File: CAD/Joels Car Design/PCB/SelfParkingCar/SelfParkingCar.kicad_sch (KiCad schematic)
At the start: 13 parts, among them U1 ESP32-DevKitC

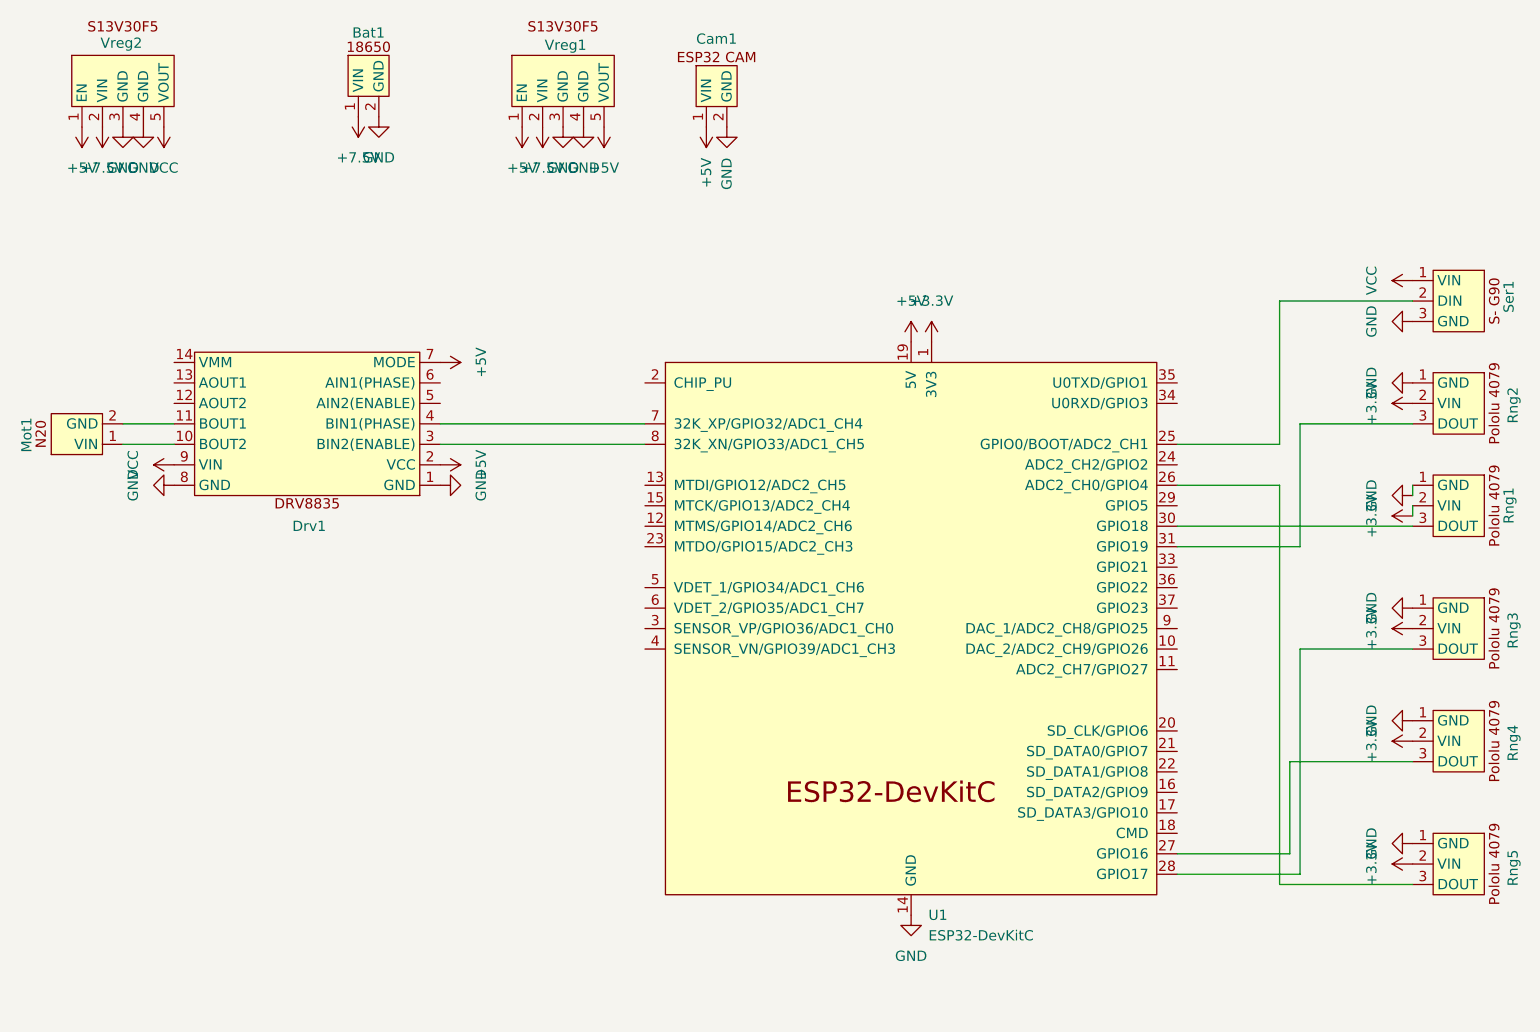
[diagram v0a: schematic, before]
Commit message: PCB Complete
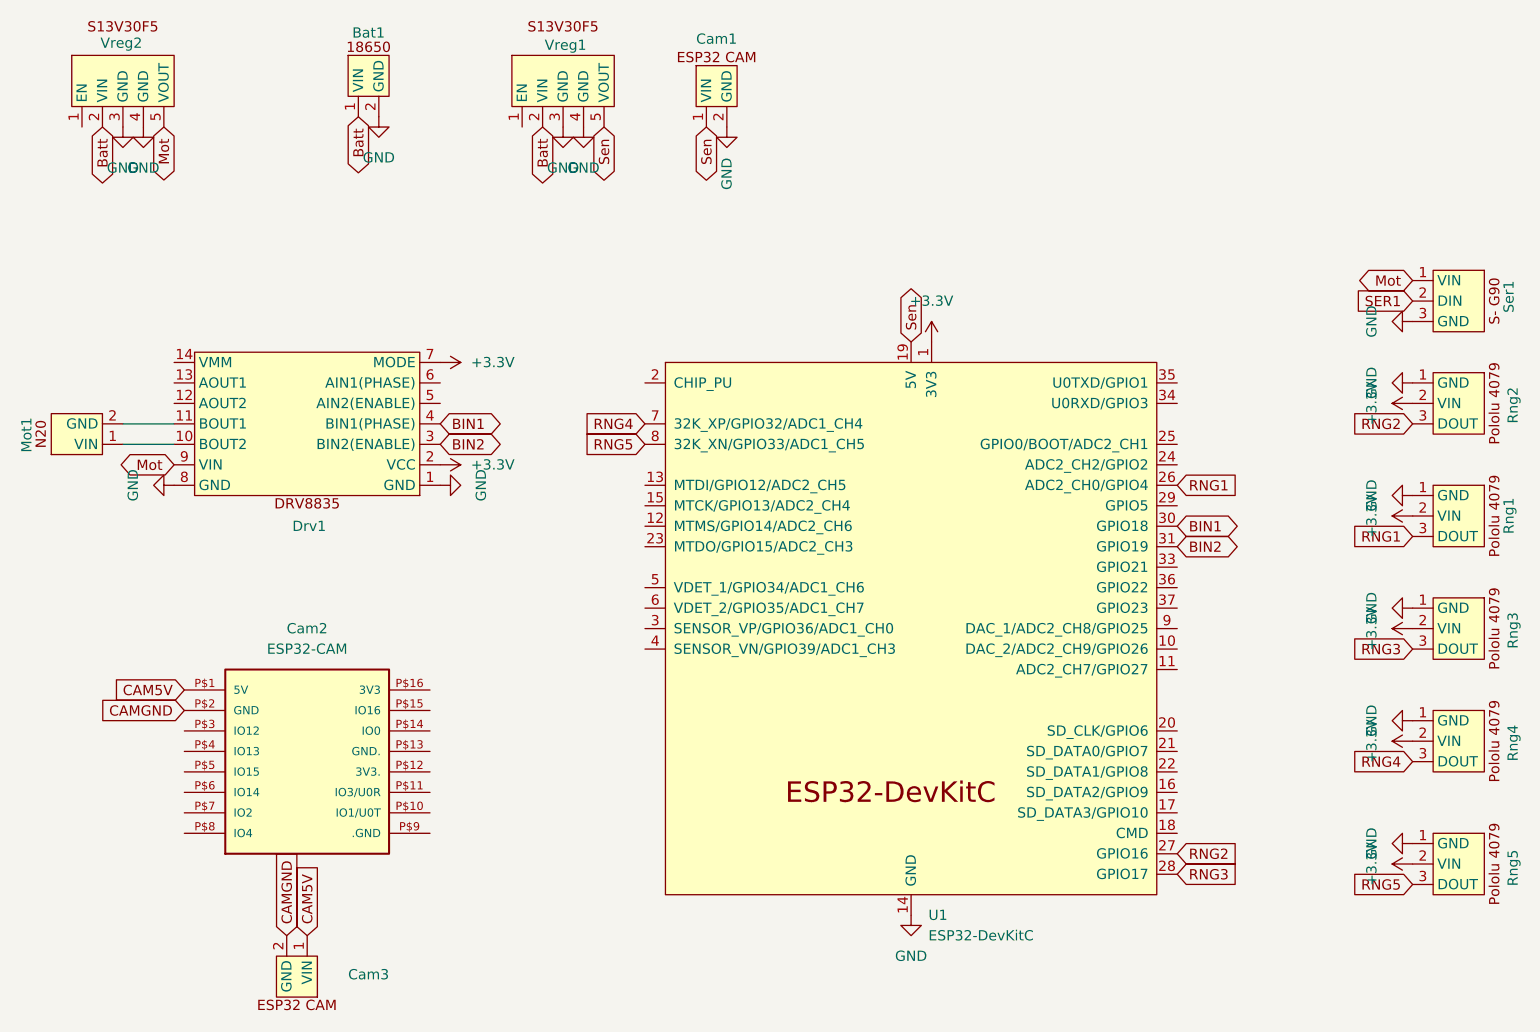
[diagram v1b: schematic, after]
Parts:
- added Cam2: ESP32-CAM, SelfParkingCar:ESP32-CAM, symbol SelfParkingCar:ESP32-CAM
- added Cam3: ~, SelfParkingCar:ESP32 Camera, symbol SelfParkingCar:ESP32 Camera
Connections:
- net +3.3V: now also Drv1.2 (VCC), Drv1.7 (MODE)
- net RNG3: now reaches Rng3.3 (DOUT), U1.28 (GPIO17)
- net at U1.25 (GPIO0/BOOT/ADC2_CH1): no longer Ser1.2 (DIN)
- net RNG1: now reaches U1.26 (ADC2_CH0/GPIO4)
- net RNG1: now also Rng1.3 (DOUT); no longer Rng5.3 (DOUT)
- net RNG2: now reaches U1.27 (GPIO16)
- net RNG2: now also Rng2.3 (DOUT); no longer Rng4.3 (DOUT)
- net BIN1: now reaches U1.30 (GPIO18)
- net BIN1: now also Drv1.4 (BIN1(PHASE)); no longer Rng1.3 (DOUT)
- net BIN2: now reaches U1.31 (GPIO19)
- net BIN2: now also Drv1.3 (BIN2(ENABLE)); no longer Rng2.3 (DOUT)
- net RNG4: now reaches U1.7 (32K_XP/GPIO32/ADC1_CH4)
- net RNG4: now also Rng4.3 (DOUT); no longer Drv1.4 (BIN1(PHASE))
- net RNG5: now reaches U1.8 (32K_XN/GPIO33/ADC1_CH5)
- net RNG5: now also Rng5.3 (DOUT); no longer Drv1.3 (BIN2(ENABLE))
- removed net +5V: Cam1.1 (VIN), Drv1.2 (VCC), Drv1.7 (MODE), U1.19 (5V), Vreg1.1 (EN), Vreg1.5 (VOUT), Vreg2.1 (EN)
- net +7.5V renamed Batt
- net VCC renamed Mot
- new net CAM5V: Cam2.P$1 (5V), Cam3.1 (VIN)
- new net CAMGND: Cam2.P$2 (GND), Cam3.2 (GND)
- new net SER1: Ser1.2 (DIN)
- new net Sen: Cam1.1 (VIN), U1.19 (5V), Vreg1.5 (VOUT)
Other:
- moved on the sheet: Rng1
